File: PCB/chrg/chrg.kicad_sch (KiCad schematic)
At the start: 19 parts, among them U1 10k, U2 CH224K, U3 IP6518, U4 220uF

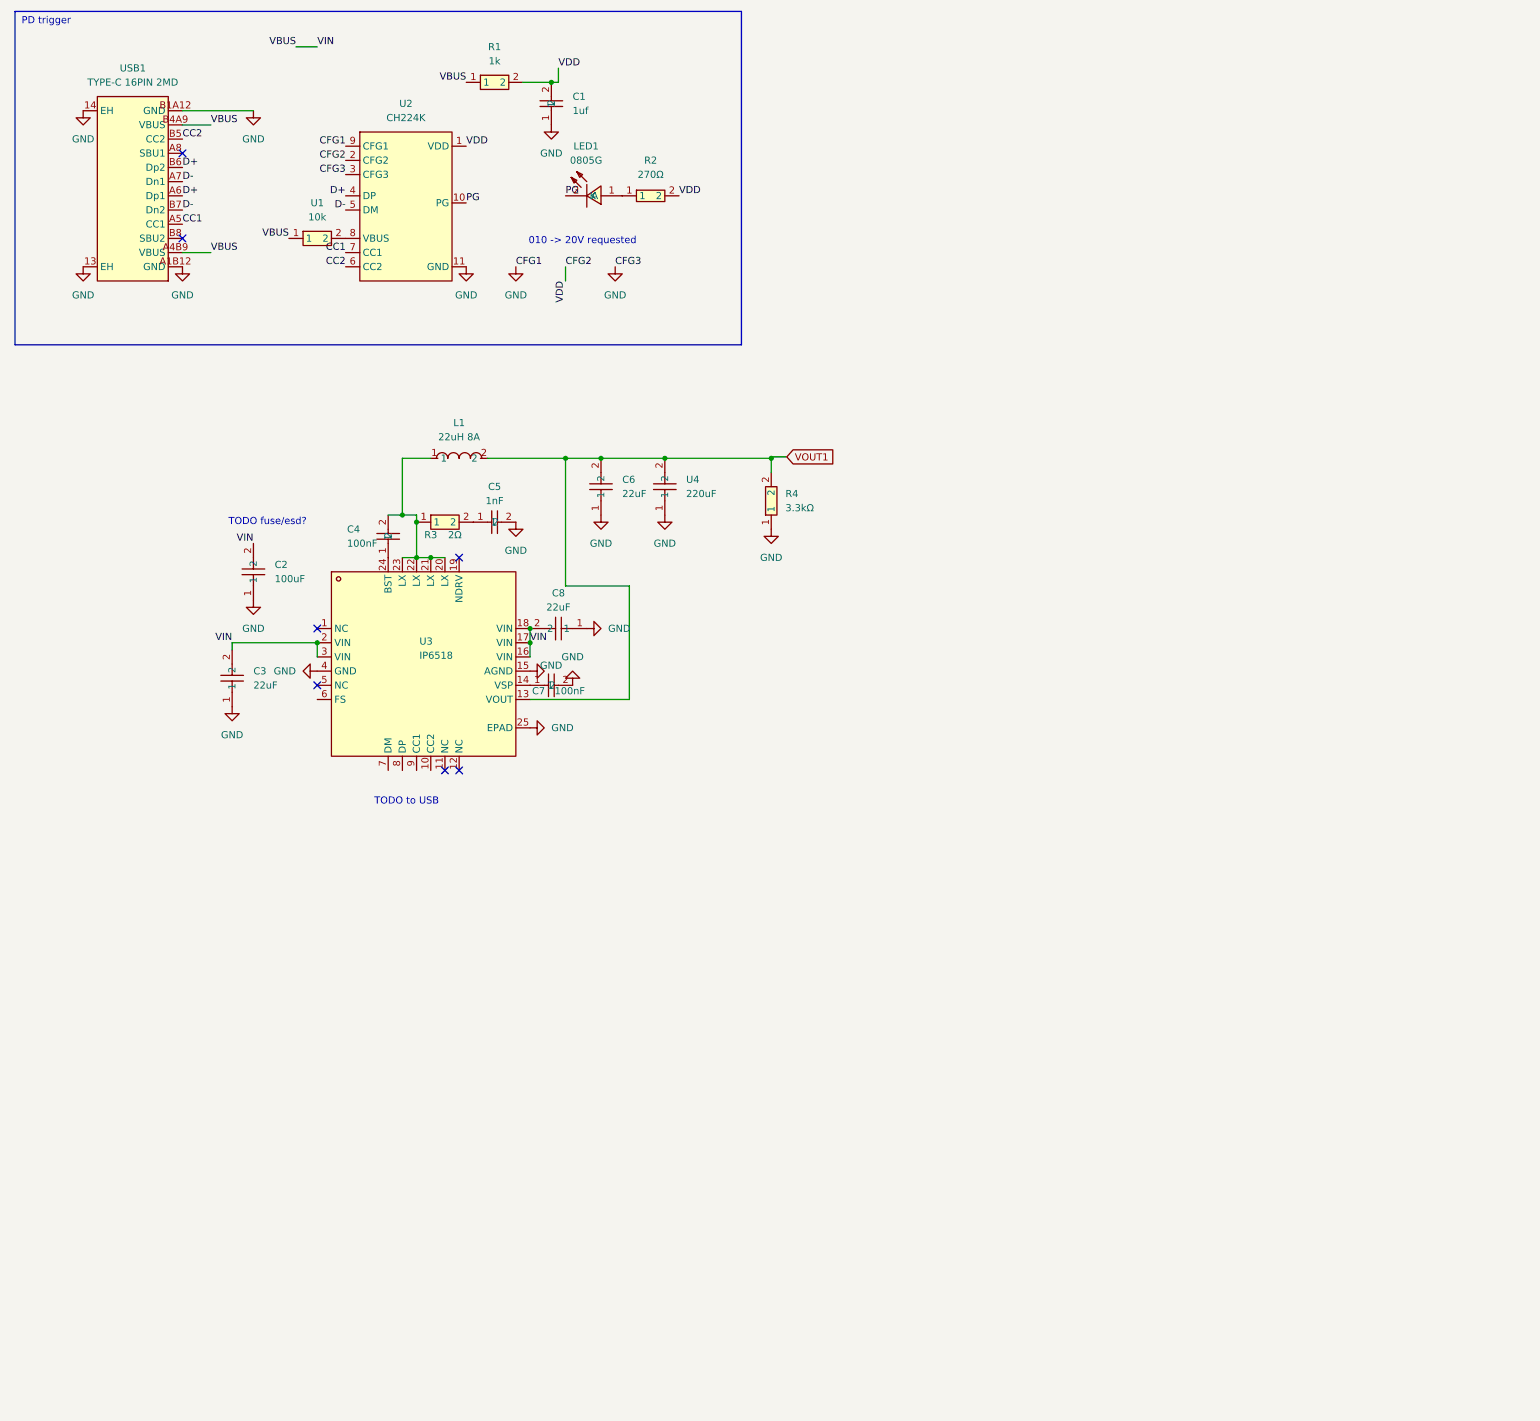
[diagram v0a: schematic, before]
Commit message: schem "done"
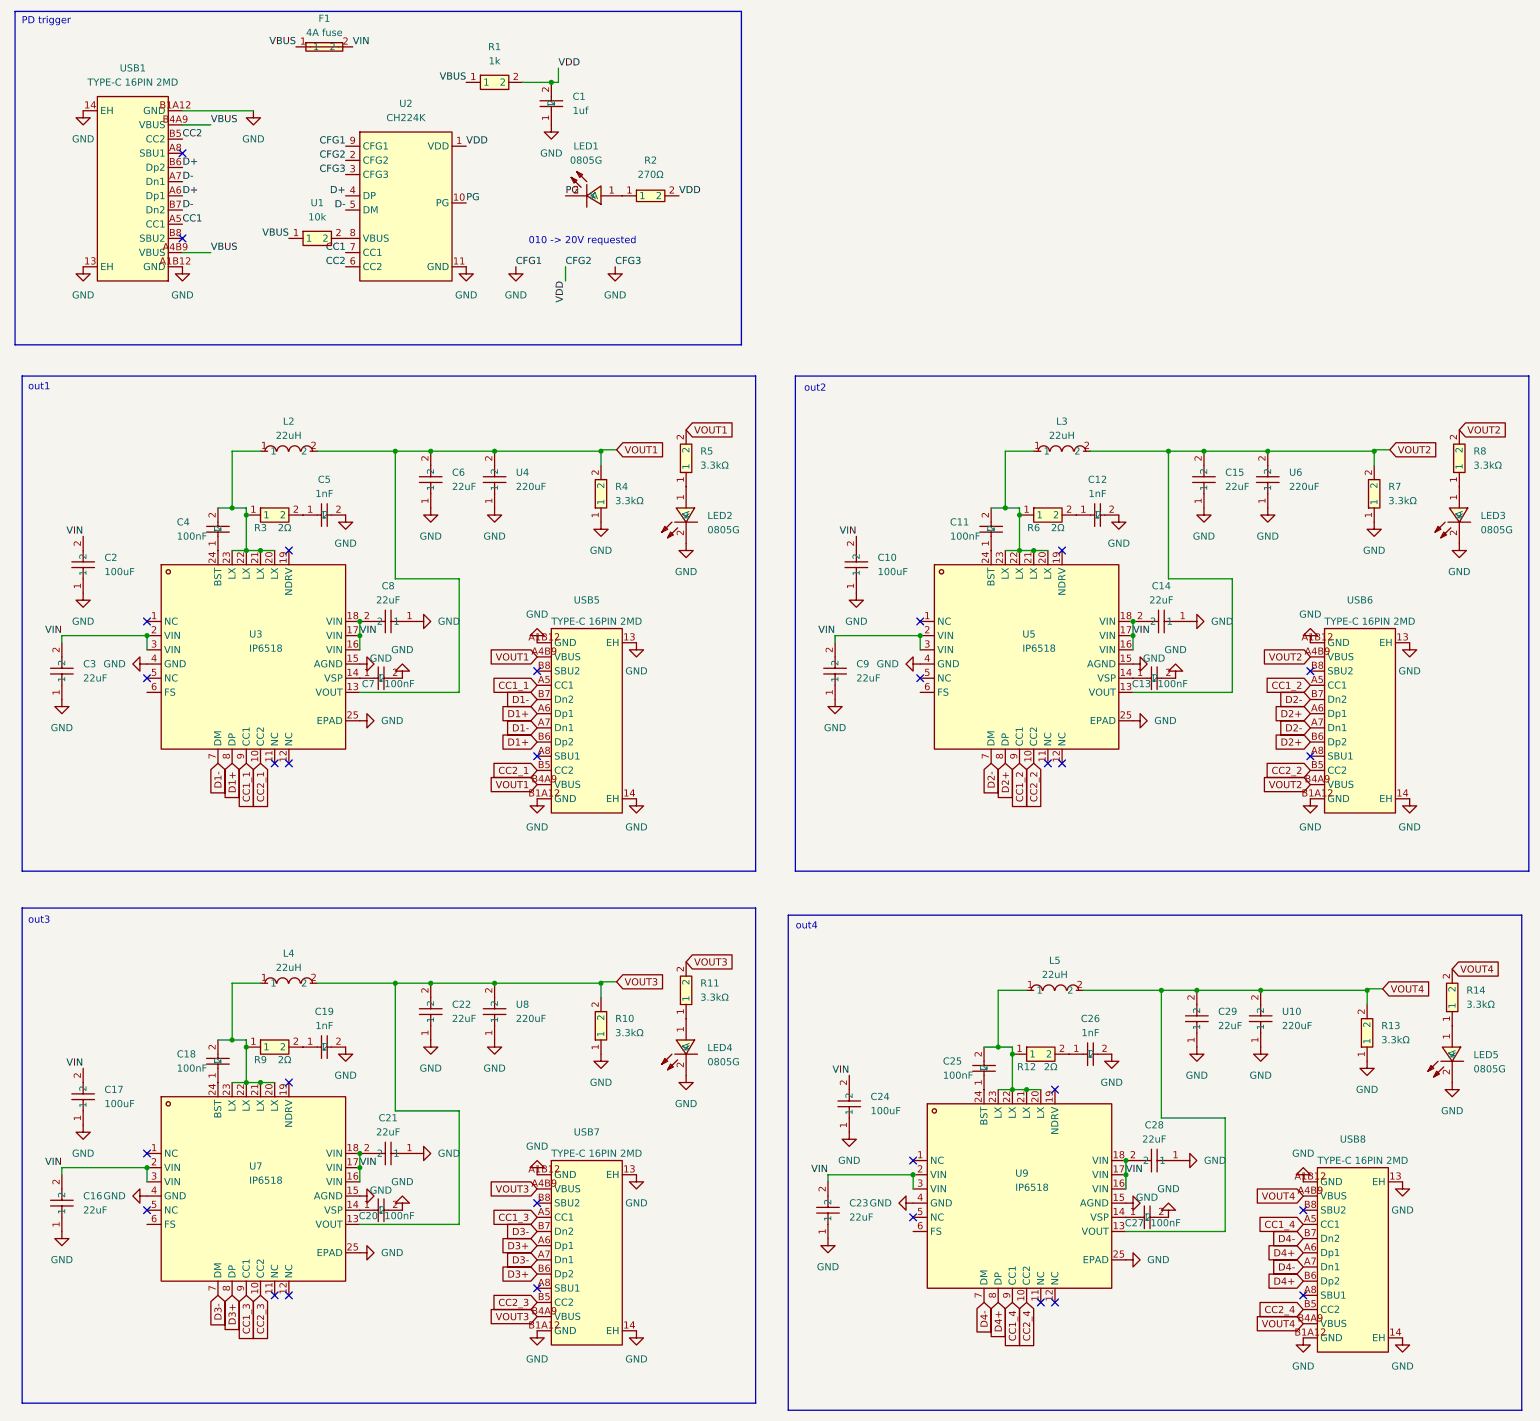
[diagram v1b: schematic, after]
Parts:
- removed L1: 22uH 8A, easyeda2kicad:IND-SMD_L13.8-W12.6_SMMS1360, symbol lcsc:SMMS1360-220M_C6849488
- added C10, C17, C24: 100uF, easyeda2kicad:C0805, symbol lcsc:JMK212BBJ107MG-TE
- added C11, C13, C18, C20, C25, C27: 100nF, easyeda2kicad:C0402, symbol lcsc:CC0402KRX7R9BB104
- added C12, C19, C26: 1nF, easyeda2kicad:C0402, symbol lcsc:CL05B102KB5NNNC
- added C14, C15, C16, C21, C22, C23, C28, C29, C9: 22uF, easyeda2kicad:C0402, symbol lcsc:CGA0402X5R226M6R3GT
- added F1: 4A fuse, easyeda2kicad:FUSE-SMD_2410-T4A-125V, symbol lcsc:2410T4A_125V
- added L2, L3, L4, L5: 22uH, easyeda2kicad:IND-SMD_L18.3-W18.2_MTF1810, symbol lcsc:MTF1810-220M
- added LED2, LED3, LED4, LED5: 0805G, lcsc:LED0805-R-RD, symbol lcsc:0805G
- added R10, R11, R13, R14, R5, R7, R8: 3.3kΩ, easyeda2kicad:R0402, symbol lcsc:RC0402FR-073K3L
- added R12, R6, R9: 2Ω, easyeda2kicad:R0402, symbol lcsc:FRC0402J2R0TS
- added U10, U6, U8: 220uF, easyeda2kicad:C1206, symbol lcsc:GRM31CR60G227ME11L
- added U5, U7, U9: IP6518, easyeda2kicad:QFN-24_L4.0-W4.0-P0.50-BL-EP2.6, symbol lcsc:IP6518
- added USB5, USB6, USB7, USB8: TYPE-C 16PIN 2MD, lcsc:USB-C-SMD_TYPE-C-16PIN-2MD-073, symbol lcsc:TYPE-C16PIN2MD
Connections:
- net GND: now also C10.1, C12.2, C13.2, C14.1, C15.1, C16.1, C17.1, C19.2, C20.2, C21.1, C22.1, C23.1, C24.1, C26.2, C27.2, C28.1, C29.1, C9.1, LED2.2 (K), LED3.2 (K), LED4.2 (K), LED5.2 (K), R10.1, R13.1, R7.1, U10.1, U5.15 (AGND), U5.25 (EPAD), U5.4 (GND), U6.1, U7.15 (AGND), U7.25 (EPAD), U7.4 (GND), U8.1, U9.15 (AGND), U9.25 (EPAD), U9.4 (GND), USB5.13 (EH), USB5.14 (EH), USB5.A1B12 (GND), USB5.B1A12 (GND), USB6.13 (EH), USB6.14 (EH), USB6.A1B12 (GND), USB6.B1A12 (GND), USB7.13 (EH), USB7.14 (EH), USB7.A1B12 (GND), USB7.B1A12 (GND), USB8.13 (EH), USB8.14 (EH), USB8.A1B12 (GND), USB8.B1A12 (GND)
- net VBUS: now also F1.1; no longer C2.2, C3.2, C8.2, U3.16 (VIN), U3.17 (VIN), U3.18 (VIN), U3.2 (VIN), U3.3 (VIN)
- net VOUT1: now also L2.2, R5.2, USB5.A4B9 (VBUS), USB5.B4A9 (VBUS)
- net at C4.2, R3.1, U3.20 (LX)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: now also L2.1
- net CC2_1: now reaches U3.10 (CC2)
- net CC2_1: now also USB5.B5 (CC2)
- net D1-: now reaches U3.7 (DM)
- net D1-: now also USB5.A7 (Dn1), USB5.B7 (Dn2)
- net D1+: now reaches U3.8 (DP)
- net D1+: now also USB5.A6 (Dp1), USB5.B6 (Dp2)
- net CC1_1: now reaches U3.9 (CC1)
- net CC1_1: now also USB5.A5 (CC1)
- new net: LED2.1 (A), R5.1
- new net: C25.1, U9.24 (BST)
- new net: C25.2, L5.1, R12.1, U9.20 (LX), U9.21 (LX), U9.22 (LX), U9.23 (LX)
- new net: C11.2, L3.1, R6.1, U5.20 (LX), U5.21 (LX), U5.22 (LX), U5.23 (LX)
- new net: C12.1, R6.2
- new net: LED5.1 (A), R14.1
- new net: C26.1, R12.2
- new net: LED4.1 (A), R11.1
- new net: C18.1, U7.24 (BST)
- new net: C18.2, L4.1, R9.1, U7.20 (LX), U7.21 (LX), U7.22 (LX), U7.23 (LX)
- new net: C20.1, U7.14 (VSP)
- new net: C13.1, U5.14 (VSP)
- new net: LED3.1 (A), R8.1
- new net: C19.1, R9.2
- new net: C11.1, U5.24 (BST)
- new net: C27.1, U9.14 (VSP)
- new net CC1_2: U5.9 (CC1), USB6.A5 (CC1)
- new net CC1_3: U7.9 (CC1), USB7.A5 (CC1)
- new net CC1_4: U9.9 (CC1), USB8.A5 (CC1)
- new net CC2_2: U5.10 (CC2), USB6.B5 (CC2)
- new net CC2_3: U7.10 (CC2), USB7.B5 (CC2)
- new net CC2_4: U9.10 (CC2), USB8.B5 (CC2)
- new net D2+: U5.8 (DP), USB6.A6 (Dp1), USB6.B6 (Dp2)
- new net D2-: U5.7 (DM), USB6.A7 (Dn1), USB6.B7 (Dn2)
- new net D3+: U7.8 (DP), USB7.A6 (Dp1), USB7.B6 (Dp2)
- new net D3-: U7.7 (DM), USB7.A7 (Dn1), USB7.B7 (Dn2)
- new net D4+: U9.8 (DP), USB8.A6 (Dp1), USB8.B6 (Dp2)
- new net D4-: U9.7 (DM), USB8.A7 (Dn1), USB8.B7 (Dn2)
- new net VIN: C10.2, C14.2, C16.2, C17.2, C2.2, C21.2, C23.2, C24.2, C28.2, C3.2, C8.2, C9.2, F1.2, U3.16 (VIN), U3.17 (VIN), U3.18 (VIN), U3.2 (VIN), U3.3 (VIN), U5.16 (VIN), U5.17 (VIN), U5.18 (VIN), U5.2 (VIN), U5.3 (VIN), U7.16 (VIN), U7.17 (VIN), U7.18 (VIN), U7.2 (VIN), U7.3 (VIN), U9.16 (VIN), U9.17 (VIN), U9.18 (VIN), U9.2 (VIN), U9.3 (VIN)
- new net VOUT2: C15.2, L3.2, R7.2, R8.2, U5.13 (VOUT), U6.2, USB6.A4B9 (VBUS), USB6.B4A9 (VBUS)
- new net VOUT3: C22.2, L4.2, R10.2, R11.2, U7.13 (VOUT), U8.2, USB7.A4B9 (VBUS), USB7.B4A9 (VBUS)
- new net VOUT4: C29.2, L5.2, R13.2, R14.2, U10.2, U9.13 (VOUT), USB8.A4B9 (VBUS), USB8.B4A9 (VBUS)
- no-connect marks 7 -> 30
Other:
- note added: "out1"
- note added: "out2"
- note added: "out3"
- note added: "out4"
- note removed: "TODO fuse/esd?"
- note removed: "TODO to USB"
- moved on the sheet: C2, C3, C4, C5, C6, C7, C8, R3, R4, U3, U4
